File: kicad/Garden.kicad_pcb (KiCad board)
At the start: 2 copper layers, 55.9 x 58.4 mm, 24 parts, among them J1 EC, J10 FAN_PWM, J11 SPI, J2 TEMP, J3 DHT, J4 PH, J5 Serial, J6 Power, J7 RELAIS, J8 RC, J9 LCD, SW1 SW_Push, SW2 SW_Push, SW3 SW_Push, SW4 SW_Push, SW5 SW_Push

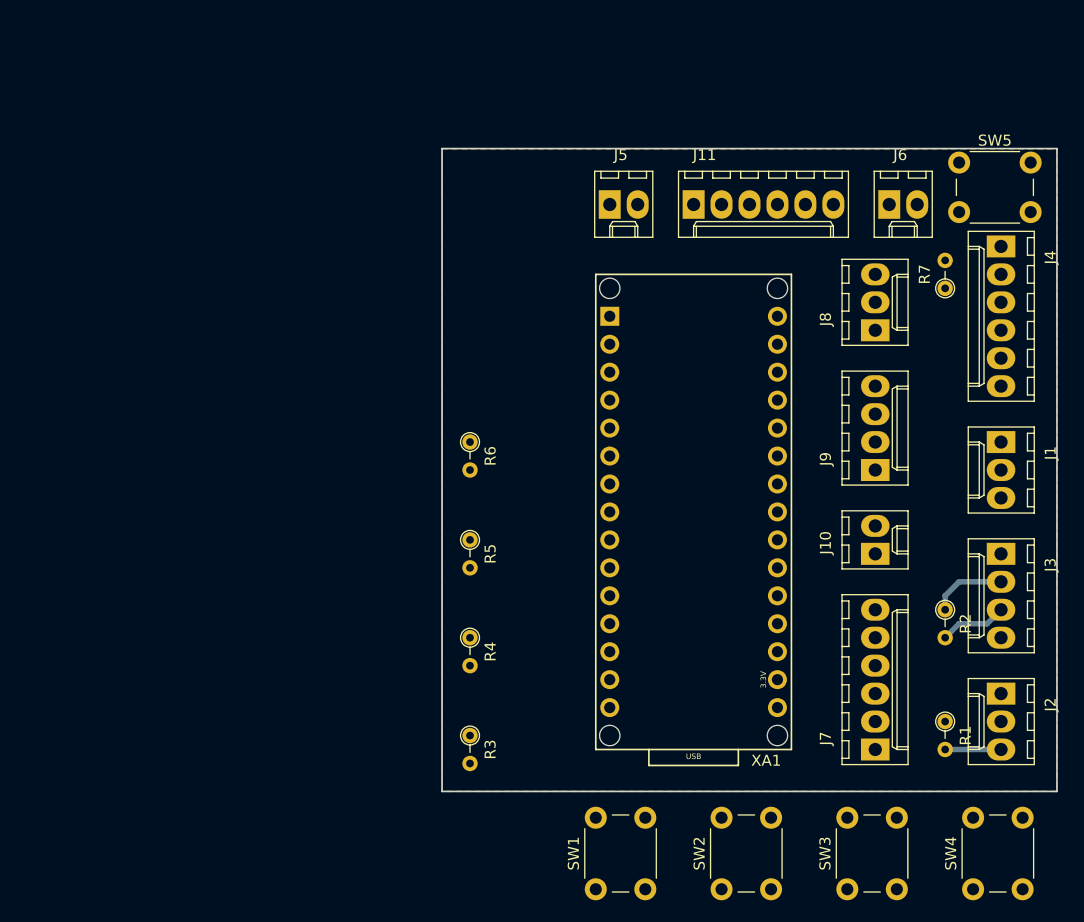
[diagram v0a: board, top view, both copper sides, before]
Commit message: New pcb design with butons, wip
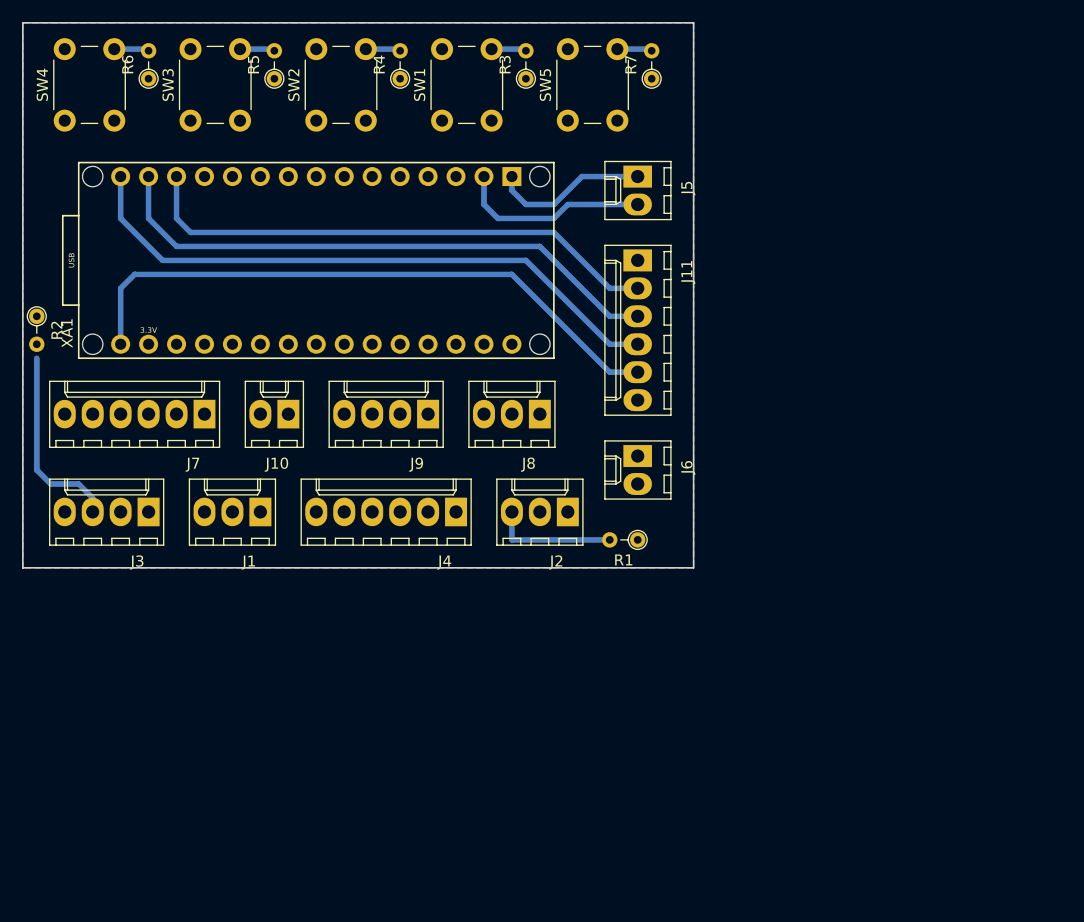
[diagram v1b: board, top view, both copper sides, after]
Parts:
- moved SW4 108.1 mm to (88.9, 48.3)
- moved SW3 91.9 mm to (100.3, 48.3)
- moved R2 86.8 mm to (86.4, 66.0)
- moved SW2 79.0 mm to (111.8, 48.3)
- moved J3 77.6 mm to (96.5, 83.8), turned to 180 degrees
- moved XA1 71.4 mm to (90.2, 61.0), turned to 270 degrees
- moved SW1 71.2 mm to (123.2, 48.3)
- moved J7 68.2 mm to (101.6, 74.9), turned to 180 degrees
- moved J1 67.6 mm to (106.7, 83.8), turned to 180 degrees
- moved R3 59.9 mm to (130.8, 44.5), turned to 90 degrees
- moved J4 55.1 mm to (124.5, 83.8), turned to 180 degrees
- moved J10 54.8 mm to (109.2, 74.9), turned to 180 degrees
- moved R4 51.2 mm to (119.4, 44.5), turned to 90 degrees
- moved R5 45.5 mm to (108.0, 44.5), turned to 90 degrees
- moved R6 44.1 mm to (96.5, 44.5), turned to 90 degrees
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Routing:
- net D13_SCK: track 0.00 -> 59.5 mm
- net D12_MISO: track 0.00 -> 58.7 mm
- net D11_MOSI: track 0.00 -> 55.1 mm
- net D10_CS: track 0.00 -> 52.8 mm
- net RX: track 0.00 -> 17.6 mm
- net TX: track 0.00 -> 14.3 mm
- net Net-(J3-Pad3): track 6.13 -> 17.6 mm
- net A0: track 6.88 -> 0.00 mm
- net D3: track 5.08 -> 11.4 mm
- net D2: track 0.00 -> 3.18 mm
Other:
- board size 55.9 x 58.4 mm -> 61 x 49.5 mm
